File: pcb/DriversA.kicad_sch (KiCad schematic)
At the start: 49 parts, among them J13 54202-S0806ALF, J14 54202-S0806ALF, J5 TERM BLOCK, J6 TERM BLOCK, Q6 BSS84, Q7 BSS84, U3 TAS5720MRSMR, U4 TAS5720MRSMR

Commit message: ADDED Grounding Structure
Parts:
- U3, U4: footprint symbols_footprints:VQFN32_RSM0032B -> symbols_footprints:VQFN32_RSM0032B_NV
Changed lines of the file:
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@@
 			)
 		)
-		(property "Footprint" "symbols_footprints:VQFN32_RSM0032B"
+		(property "Footprint" "symbols_footprints:VQFN32_RSM0032B_NV"
 			(at 218.44 113.03 0)
 			(effects
@@
 			)
 		)
-		(property "Footprint" "symbols_footprints:VQFN32_RSM0032B"
+		(property "Footprint" "symbols_footprints:VQFN32_RSM0032B_NV"
 			(at 101.6 57.15 0)
 			(effects

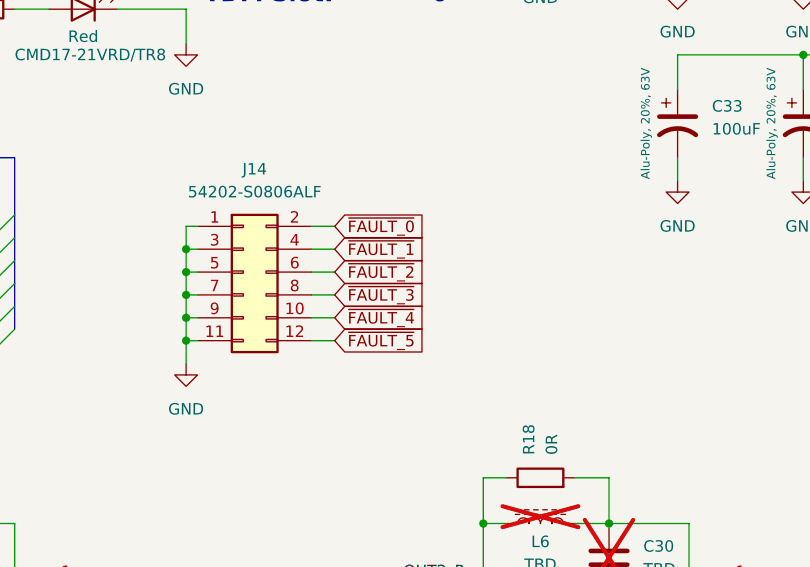
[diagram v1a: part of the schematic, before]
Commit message: DONE Routing first two drivers
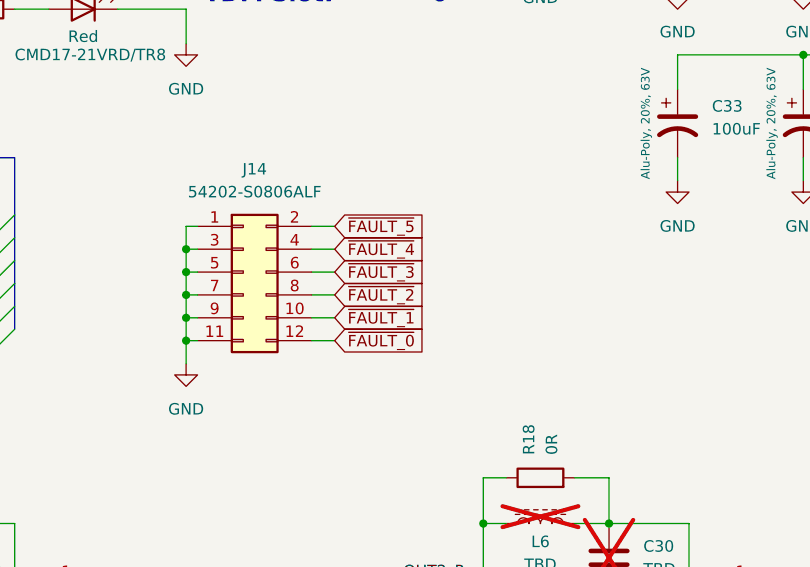
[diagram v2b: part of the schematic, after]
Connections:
- net ~{FAULT_0}: now also J14.12 (Pin_12); no longer J14.2 (Pin_2)
- net ~{FAULT_1}: now also J14.10 (Pin_10); no longer J14.4 (Pin_4)
- net ~{FAULT_2}: now also J14.8 (Pin_8); no longer J14.6 (Pin_6)
- net ~{FAULT_3}: now also J14.6 (Pin_6); no longer J14.8 (Pin_8)
- net ~{FAULT_4}: now also J14.4 (Pin_4); no longer J14.10 (Pin_10)
- net ~{FAULT_5}: now also J14.2 (Pin_2); no longer J14.12 (Pin_12)
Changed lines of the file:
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@@
 	(wire
 		(pts
+			(xy 99.06 137.16) (xy 101.6 137.16)
+		)
+		(stroke
+			(width 0)
+			(type default)
+		)
+	)
+	(wire
+		(pts
 			(xy 240.03 118.11) (xy 250.19 118.11)
 		)
@@
 	(wire
 		(pts
-			(xy 99.06 137.16) (xy 101.6 137.16)
-		)
-		(stroke
-			(width 0)
-			(type default)
-		)
-	)
-	(wire
-		(pts
 			(xy 124.46 85.09) (xy 124.46 90.17)
 		)
@@
 	(wire
 		(pts
+			(xy 99.06 124.46) (xy 101.6 124.46)
+		)
+		(stroke
+			(width 0)
+			(type default)
+		)
+	)
+	(wire
+		(pts
 			(xy 124.46 77.47) (xy 124.46 80.01)
 		)
@@
 	(wire
 		(pts
-			(xy 99.06 132.08) (xy 101.6 132.08)
-		)
-		(stroke
-			(width 0)
-			(type default)
-		)
-	)
-	(wire
-		(pts
 			(xy 240.03 107.95) (xy 240.03 105.41)
 		)
@@
 	(wire
 		(pts
-			(xy 99.06 134.62) (xy 101.6 134.62)
-		)
-		(stroke
-			(width 0)
-			(type default)
-		)
-	)
-	(wire
-		(pts
 			(xy 139.7 105.41) (xy 153.67 105.41)
 		)
@@
 	(wire
 		(pts
-			(xy 99.06 124.46) (xy 101.6 124.46)
-		)
-		(stroke
-			(width 0)
-			(type default)
-		)
-	)
-	(wire
-		(pts
 			(xy 43.18 163.83) (xy 43.18 157.48)
 		)
@@
 		)
 	)
-	(wire
+	(bus
 		(pts
-			(xy 99.06 129.54) (xy 101.6 129.54)
+			(xy 72.39 52.07) (xy 72.39 54.61)
 		)
 		(stroke
@@
 		)
 	)
-	(bus
+	(wire
 		(pts
-			(xy 72.39 52.07) (xy 72.39 54.61)
+			(xy 238.76 105.41) (xy 240.03 105.41)
 		)
 		(stroke
@@
 	(wire
 		(pts
-			(xy 238.76 105.41) (xy 240.03 105.41)
+			(xy 99.06 129.54) (xy 101.6 129.54)
 		)
 		(stroke
@@
 	(wire
 		(pts
+			(xy 99.06 127) (xy 101.6 127)
+		)
+		(stroke
+			(width 0)
+			(type default)
+		)
+	)
+	(wire
+		(pts
 			(xy 74.93 54.61) (xy 81.28 54.61)
 		)
@@
 	(wire
 		(pts
+			(xy 99.06 134.62) (xy 101.6 134.62)
+		)
+		(stroke
+			(width 0)
+			(type default)
+		)
+	)
+	(wire
+		(pts
 			(xy 241.3 128.27) (xy 241.3 133.35)
 		)
@@
 		)
 	)
+	(wire
+		(pts
+			(xy 99.06 132.08) (xy 101.6 132.08)
+		)
+		(stroke
+			(width 0)
+			(type default)
+		)
+	)
 	(bus
 		(pts
@@
 	(wire
 		(pts
-			(xy 99.06 127) (xy 101.6 127)
-		)
-		(stroke
-			(width 0)
-			(type default)
-		)
-	)
-	(wire
-		(pts
 			(xy 241.3 133.35) (xy 241.3 135.89)
 		)
@@
 	(global_label "~{FAULT_4}"
 		(shape input)
-		(at 101.6 134.62 0)
+		(at 101.6 127 0)
 		(fields_autoplaced yes)
 		(effects
@@
 		)
 		(property "Intersheetrefs" "${INTERSHEET_REFS}"
-			(at 111.7316 134.62 0)
+			(at 111.7316 127 0)
 			(effects
 				(font
@@
 	(global_label "~{FAULT_0}"
 		(shape input)
-		(at 101.6 124.46 0)
+		(at 101.6 137.16 0)
 		(fields_autoplaced yes)
 		(effects
@@
 		)
 		(property "Intersheetrefs" "${INTERSHEET_REFS}"
-			(at 111.7316 124.46 0)
+			(at 111.7316 137.16 0)
 			(effects
 				(font
@@
 	(global_label "~{FAULT_5}"
 		(shape input)
-		(at 101.6 137.16 0)
+		(at 101.6 124.46 0)
 		(fields_autoplaced yes)
 		(effects
@@
 		)
 		(property "Intersheetrefs" "${INTERSHEET_REFS}"
-			(at 111.7316 137.16 0)
+			(at 111.7316 124.46 0)
 			(effects
 				(font
@@
 	(global_label "~{FAULT_2}"
 		(shape input)
-		(at 101.6 129.54 0)
+		(at 101.6 132.08 0)
 		(fields_autoplaced yes)
 		(effects
@@
 		)
 		(property "Intersheetrefs" "${INTERSHEET_REFS}"
-			(at 111.7316 129.54 0)
+			(at 111.7316 132.08 0)
 			(effects
 				(font
@@
 	(global_label "~{FAULT_1}"
 		(shape input)
-		(at 101.6 127 0)
+		(at 101.6 134.62 0)
 		(fields_autoplaced yes)
 		(effects
@@
 		)
 		(property "Intersheetrefs" "${INTERSHEET_REFS}"
-			(at 111.7316 127 0)
+			(at 111.7316 134.62 0)
 			(effects
 				(font
@@
 	(global_label "~{FAULT_3}"
 		(shape input)
-		(at 101.6 132.08 0)
+		(at 101.6 129.54 0)
 		(fields_autoplaced yes)
 		(effects
@@
 		)
 		(property "Intersheetrefs" "${INTERSHEET_REFS}"
-			(at 111.7316 132.08 0)
+			(at 111.7316 129.54 0)
 			(effects
 				(font
